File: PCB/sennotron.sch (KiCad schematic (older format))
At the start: 7 parts

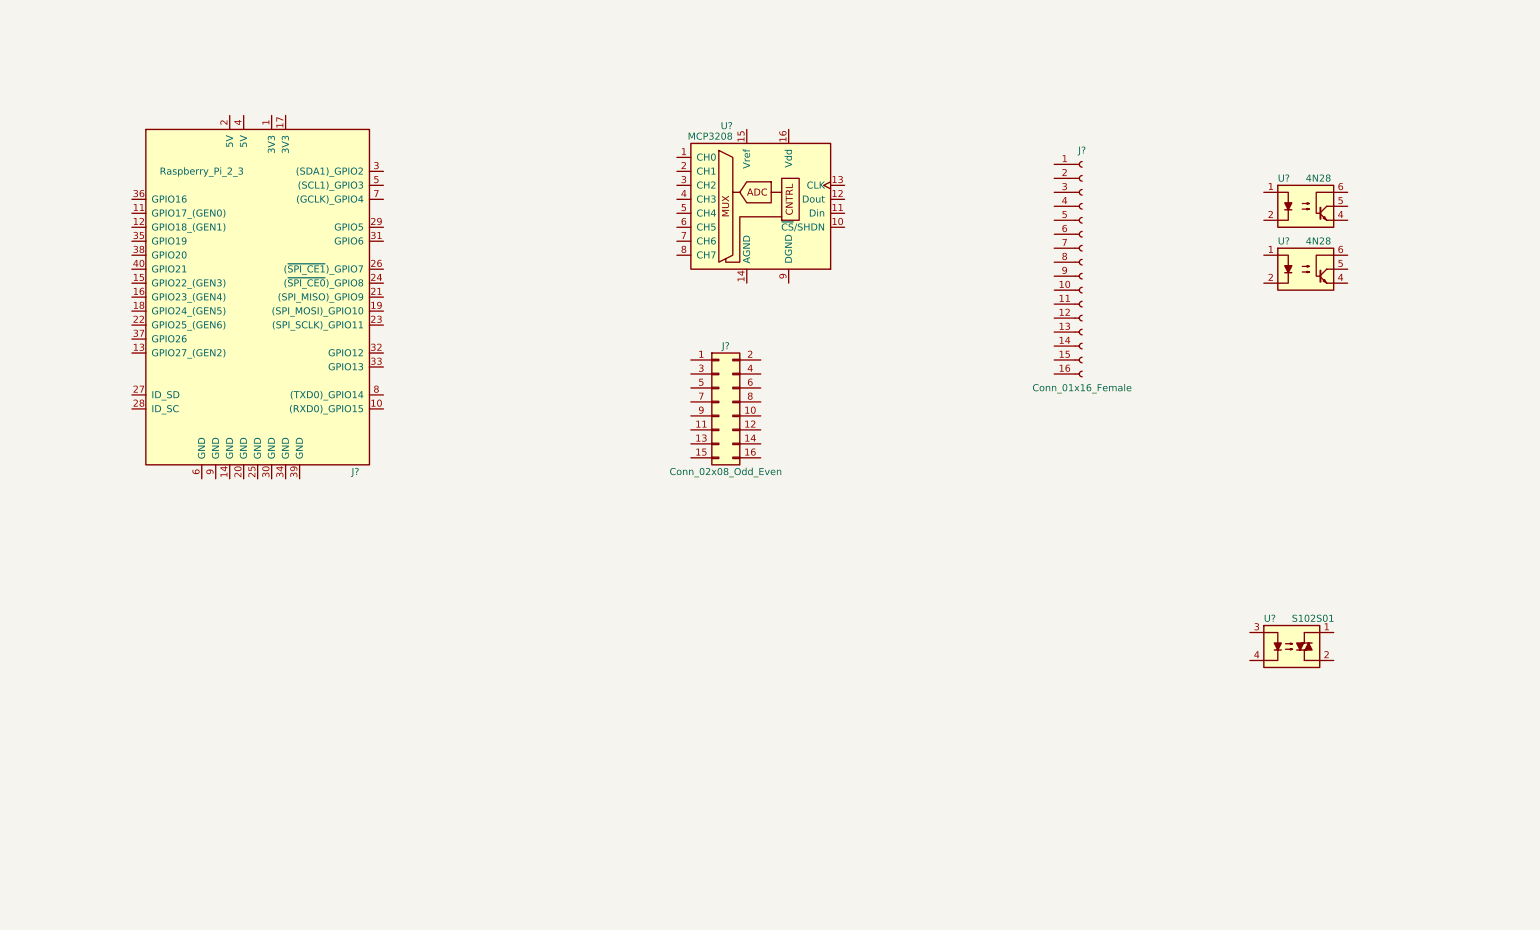
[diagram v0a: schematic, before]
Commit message: Schematics and PCB design updated
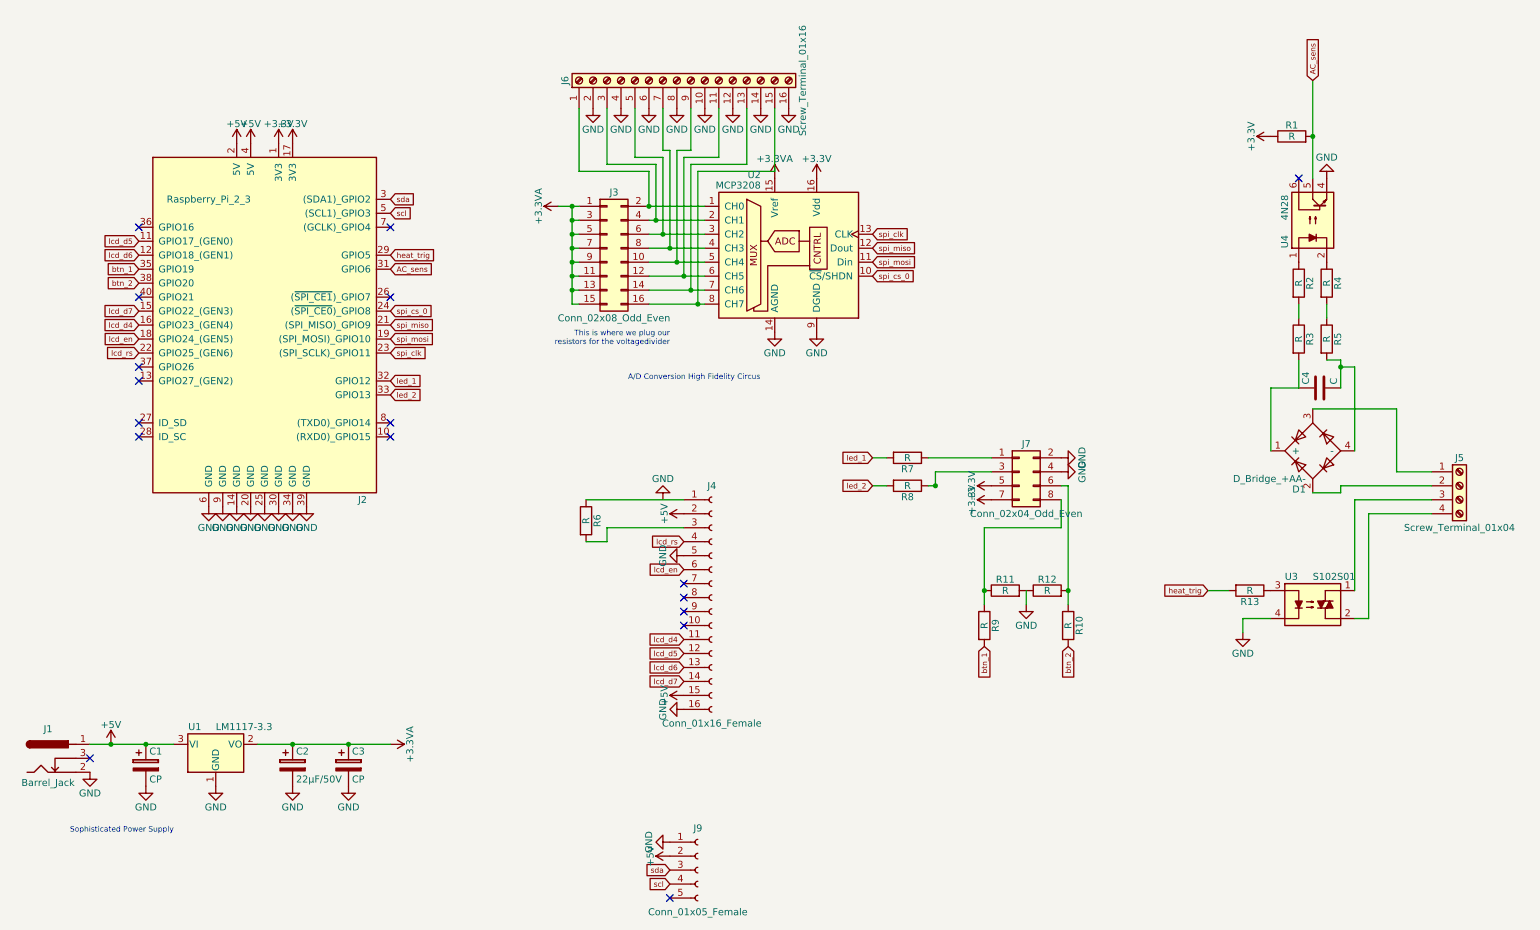
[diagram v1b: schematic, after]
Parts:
- removed J?: Raspberry_Pi_2_3, Pin_Headers:Pin_Header_Straight_2x20, symbol Raspberry_Pi_2_3
- removed U?: 4N28, Housings_DIP:DIP-6_W7.62mm, symbol 4N28
- added C1, C3: CP, Capacitors_THT:CP_Radial_D8.0mm_P5.00mm, symbol CP
- added C2: 22µF/50V, Capacitors_THT:CP_Radial_D8.0mm_P5.00mm, symbol CP
- added C4: C, Capacitors_SMD:C_2220_HandSoldering, symbol C
- added D1: D_Bridge_+AA-, custom:CUI-PJ-102A_dc-barrel-jack, symbol D_Bridge_+AA-
- added J1: Barrel_Jack, Connectors:BARREL_JACK, symbol Barrel_Jack
- added J2: Raspberry_Pi_2_3, Pin_Headers:Pin_Header_Straight_2x20_Pitch2.54mm, symbol Raspberry_Pi_2_3
- added J5: Screw_Terminal_01x04, TerminalBlocks_Phoenix:TerminalBlock_Phoenix_PT-3.5mm_4pol, symbol Screw_Terminal_01x04
- added J6: Screw_Terminal_01x16, TerminalBlocks_Phoenix:TerminalBlock_Phoenix_PT-3.5mm_16pol, symbol Screw_Terminal_01x16
- added J7: Conn_02x04_Odd_Even, Pin_Headers:Pin_Header_Straight_2x04_Pitch2.54mm, symbol Conn_02x04_Odd_Even
- added J9: Conn_01x05_Female, Socket_Strips:Socket_Strip_Straight_1x05_Pitch2.54mm, symbol Conn_01x05_Female
- added R1, R10, R11, R12, R13, R2, R3, R4, R5, R6, R7, R8, R9: R, Resistors_THT:R_Axial_DIN0207_L6.3mm_D2.5mm_P10.16mm_Horizontal, symbol R
- added U1: LM1117-3.3, Power_Integrations:TO-220, symbol LM1117-3.3
- J3: renamed from J?; footprint (none) -> Pin_Headers:Pin_Header_Straight_2x08_Pitch2.54mm
- J4: renamed from J?; footprint (none) -> Pin_Headers:Pin_Header_Straight_1x16_Pitch2.54mm
- U2: renamed from U?; footprint (none) -> Housings_DIP:DIP-16_W7.62mm_Socket
- gave numbers to parts that had none: 2
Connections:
- net at U2.1 (CH0): now also J3.2 (Pin_2), J6.1 (Pin_1)
- net spi_cs_0: now reaches U2.10 (~CS~/SHDN)
- net spi_cs_0: now also J2.24 ((~SPI_CE0~)_GPIO8)
- net spi_mosi: now reaches U2.11 (Din)
- net spi_mosi: now also J2.19 ((SPI_MOSI)_GPIO10)
- net spi_miso: now reaches U2.12 (Dout)
- net spi_miso: now also J2.21 ((SPI_MISO)_GPIO9)
- net spi_clk: now reaches U2.13 (CLK)
- net spi_clk: now also J2.23 ((SPI_SCLK)_GPIO11)
- net GND: now reaches U2.14 (AGND)
- net GND: now also J4.16 (Pin_16), J4.5 (Pin_5), U2.9 (DGND), U3.4, U4.4, C1.2, C2.2, C3.2, J1.2, J2.14 (GND), J2.20 (GND), J2.25 (GND), J2.30 (GND), J2.34 (GND), J2.39 (GND), J2.6 (GND), J2.9 (GND), J6.10 (Pin_10), J6.12 (Pin_12), J6.14 (Pin_14), J6.16 (Pin_16), J6.2 (Pin_2), J6.4 (Pin_4), J6.6 (Pin_6), J6.8 (Pin_8), J7.2 (Pin_2), J7.4 (Pin_4), J9.1 (Pin_1), R11.2, R12.1, U1.1 (GND)
- net +3.3VA: now reaches U2.15 (Vref)
- net +3.3VA: now also J3.1 (Pin_1), J3.11 (Pin_11), J3.13 (Pin_13), J3.15 (Pin_15), J3.3 (Pin_3), J3.5 (Pin_5), J3.7 (Pin_7), J3.9 (Pin_9), C2.1, C3.1, U1.2 (VO)
- net +3V3: now reaches U2.16 (Vdd)
- net +3V3: now also J2.1 (3V3), J2.17 (3V3), J7.5 (Pin_5), J7.7 (Pin_7), R1.1
- net at U2.2 (CH1): now also J3.4 (Pin_4), J6.3 (Pin_3)
- net at U2.3 (CH2): now also J3.6 (Pin_6), J6.5 (Pin_5)
- net at U2.4 (CH3): now also J3.8 (Pin_8), J6.7 (Pin_7)
- net at U2.5 (CH4): now also J3.10 (Pin_10), J6.9 (Pin_9)
- net at U2.6 (CH5): now also J3.12 (Pin_12), J6.11 (Pin_11)
- net at U2.7 (CH6): now also J3.14 (Pin_14), J6.13 (Pin_13)
- net at U2.8 (CH7): now also J3.16 (Pin_16), J6.15 (Pin_15)
- net at J4.1 (Pin_1): now also R6.1
- net lcd_d4: now reaches J4.11 (Pin_11)
- net lcd_d4: now also J2.16 (GPIO23_(GEN4))
- net lcd_d5: now reaches J4.12 (Pin_12)
- net lcd_d5: now also J2.11 (GPIO17_(GEN0))
- net lcd_d6: now reaches J4.13 (Pin_13)
- net lcd_d6: now also J2.12 (GPIO18_(GEN1))
- net lcd_d7: now reaches J4.14 (Pin_14)
- net lcd_d7: now also J2.15 (GPIO22_(GEN3))
- net +5V: now reaches J4.15 (Pin_15)
- net +5V: now also J4.2 (Pin_2), C1.1, J1.1, J2.2 (5V), J2.4 (5V), J9.2 (Pin_2), U1.3 (VI)
- net at J4.3 (Pin_3): now also R6.2
- net lcd_rs: now reaches J4.4 (Pin_4)
- net lcd_rs: now also J2.22 (GPIO25_(GEN6))
- net lcd_en: now reaches J4.6 (Pin_6)
- net lcd_en: now also J2.18 (GPIO24_(GEN5))
- net at U3.1: now also J5.3 (Pin_3)
- net at U3.2: now also J5.4 (Pin_4)
- net at U3.3: now also R13.1
- net at U4.1: now also R2.1
- net at U4.2: now also R4.1
- net AC_sens: now reaches U4.5
- net AC_sens: now also J2.31 (GPIO6), R1.2
- new net: C4.1, D1.1 (+), R3.2
- new net: C4.2, D1.4 (-), R5.2
- new net: D1.3, J5.1 (Pin_1)
- new net: D1.2, J5.2 (Pin_2)
- new net: R2.2, R3.1
- new net: R4.2, R5.1
- new net: J7.1 (Pin_1), R7.1
- new net: J7.3 (Pin_3), R8.1
- new net: J7.8 (Pin_8), R11.1, R9.1
- new net: J7.6 (Pin_6), R10.1, R12.2
- new net btn_1: J2.35 (GPIO19), R9.2
- new net btn_2: J2.38 (GPIO20), R10.2
- new net heat_trig: J2.29 (GPIO5), R13.2
- new net led_1: J2.32 (GPIO12), R7.2
- new net led_2: J2.33 (GPIO13), R8.2
- new net scl: J2.5 ((SCL1)_GPIO3), J9.4 (Pin_4)
- new net sda: J2.3 ((SDA1)_GPIO2), J9.3 (Pin_3)
- no-connect marks 0 -> 17
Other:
- note added: "A/D Conversion High Fidelity Circus"
- note added: "Sophisticated Power Supply"
- note added: "This is where we plug our\nresistors for the voltagedivider"
- moved on the sheet: J3, J4, U2, U3, U4
